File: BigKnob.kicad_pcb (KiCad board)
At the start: 2 copper layers, 45 x 80 mm, 12 parts, among them J1 NSJ12HF-1, J2 NSJ12HF-1, J3 NSJ12HF-1, J4 STEREO-JACK-SWITCHED-5-Pin, J5 STEREO-JACK-SWITCHED-5-Pin

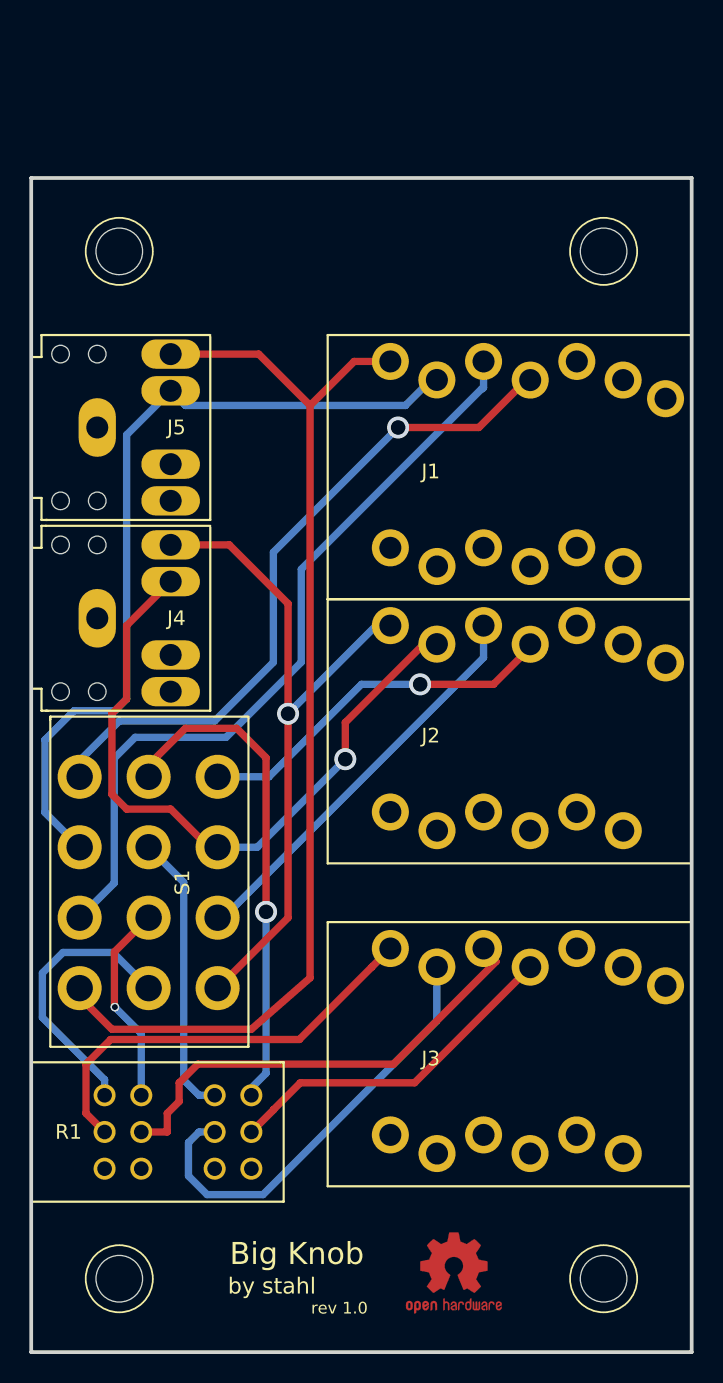
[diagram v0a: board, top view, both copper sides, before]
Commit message: :punch: v1.1
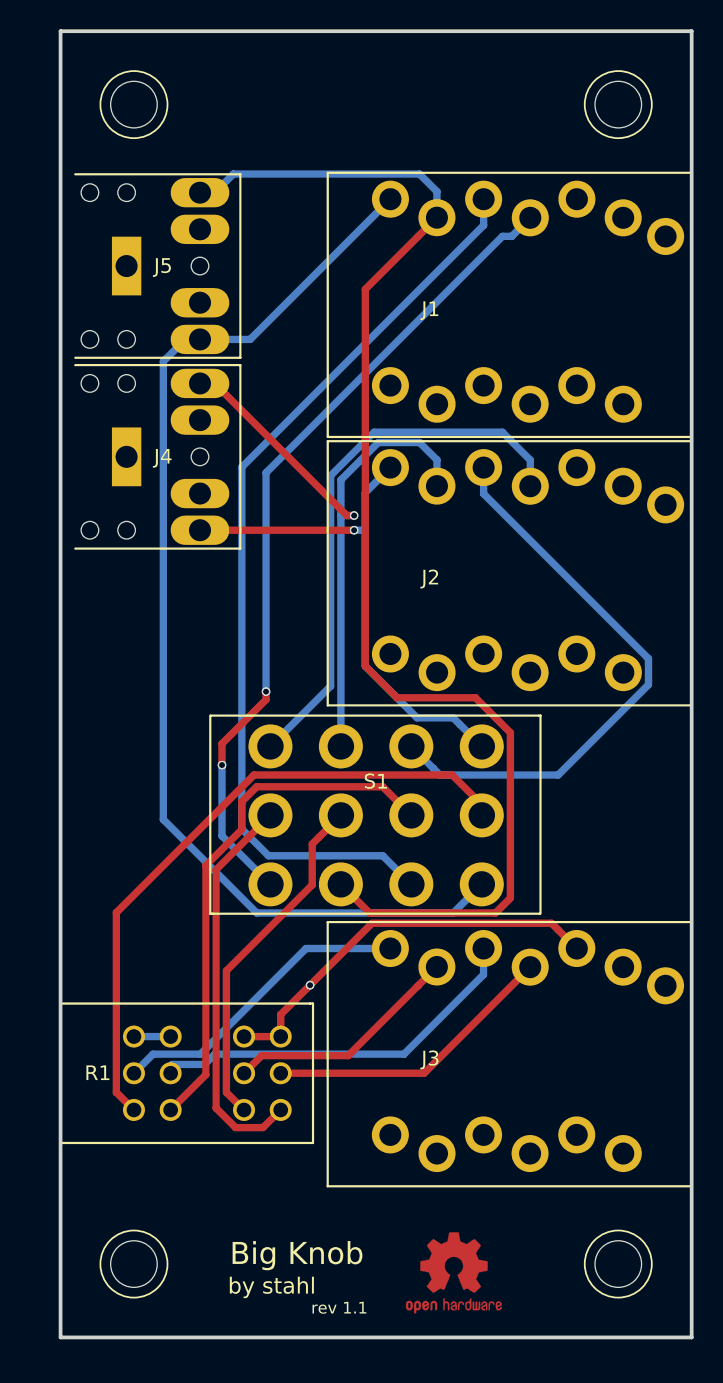
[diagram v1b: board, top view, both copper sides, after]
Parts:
- moved S1 16.2 mm to (151.8, 91.0), turned to 180 degrees
- moved J1 11.1 mm to (173.4, 56.5)
- moved J4 11.0 mm to (130.3, 66.6)
- moved J5 11.0 mm to (130.3, 53.6)
- moved J2 10.8 mm to (173.4, 74.8)
- moved REF** 10.0 mm to (168.3, 42.6)
- moved REF** 10.0 mm to (135.3, 42.6)
- moved R1 4.47 mm to (130.3, 108.6)
- moved REF** 1.41 mm to (135.3, 121.6)
- moved REF** 1.41 mm to (168.3, 121.6)
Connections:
- R1 pad A1: Net-(R1-PadA1) -> CHASSIS_GND
- R1 pad A3: CHASSIS_GND -> Net-(R1-PadA3)
- R1 pad B1: Net-(R1-PadB1) -> CHASSIS_GND
- R1 pad B3: CHASSIS_GND -> Net-(R1-PadB3)
- R1 pad C1: Net-(R1-PadC1) -> CHASSIS_GND
- R1 pad C3: CHASSIS_GND -> Net-(R1-PadC3)
- R1 pad D1: Net-(R1-PadD1) -> CHASSIS_GND
- R1 pad D3: CHASSIS_GND -> Net-(R1-PadD3)
- S1 pad 11: Net-(R1-PadD1) -> Net-(R1-PadD3)
- S1 pad 2: Net-(R1-PadA1) -> Net-(R1-PadA3)
- S1 pad 5: Net-(R1-PadB1) -> Net-(R1-PadB3)
- S1 pad 8: Net-(R1-PadC1) -> Net-(R1-PadC3)
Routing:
- net Net-(R1-PadA3): track 0.00 -> 44.3 mm
- net Net-(R1-PadB3): track 0.00 -> 35.8 mm
- net Net-(R1-PadD1): track 34.1 -> 0.00 mm, vias 1 -> 0
- net Net-(J1-Pad11): track 56.8 -> 88.0 mm
- net CHASSIS_GND: track 0.00 -> 30.5 mm, vias 0 -> 1
- net Net-(R1-PadD3): track 0.00 -> 27.7 mm
- net Net-(R1-PadC3): track 0.00 -> 23.8 mm
- net Net-(R1-PadC1): track 19.4 -> 0.00 mm
- net Net-(R1-PadA1): track 18.9 -> 0.00 mm
- net Net-(J3-Pad11): track 30.4 -> 16.1 mm
- net Net-(R1-PadB1): track 13.8 -> 0.00 mm, vias 1 -> 0
- net Net-(J2-Pad9): track 25.4 -> 38.0 mm, vias 1 -> 0
- net Net-(J2-Pad3): track 27.6 -> 39.4 mm
- net Net-(J2-Pad5): track 47.9 -> 37.3 mm
- net Net-(J1-Pad9): track 46.9 -> 57.2 mm, vias 1 -> 2
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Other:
- board size 45 x 80 mm -> 43 x 89 mm
- board text added: "2 x unbalanced stereo mini-jack input 2 x balanced stereo input balanced stereo output volume pot"
- board text added: "passive audio switch"
- board text added: "rev 1.1"
- board text removed: "rev 1.0"
